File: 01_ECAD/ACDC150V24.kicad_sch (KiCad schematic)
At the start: 0 parts

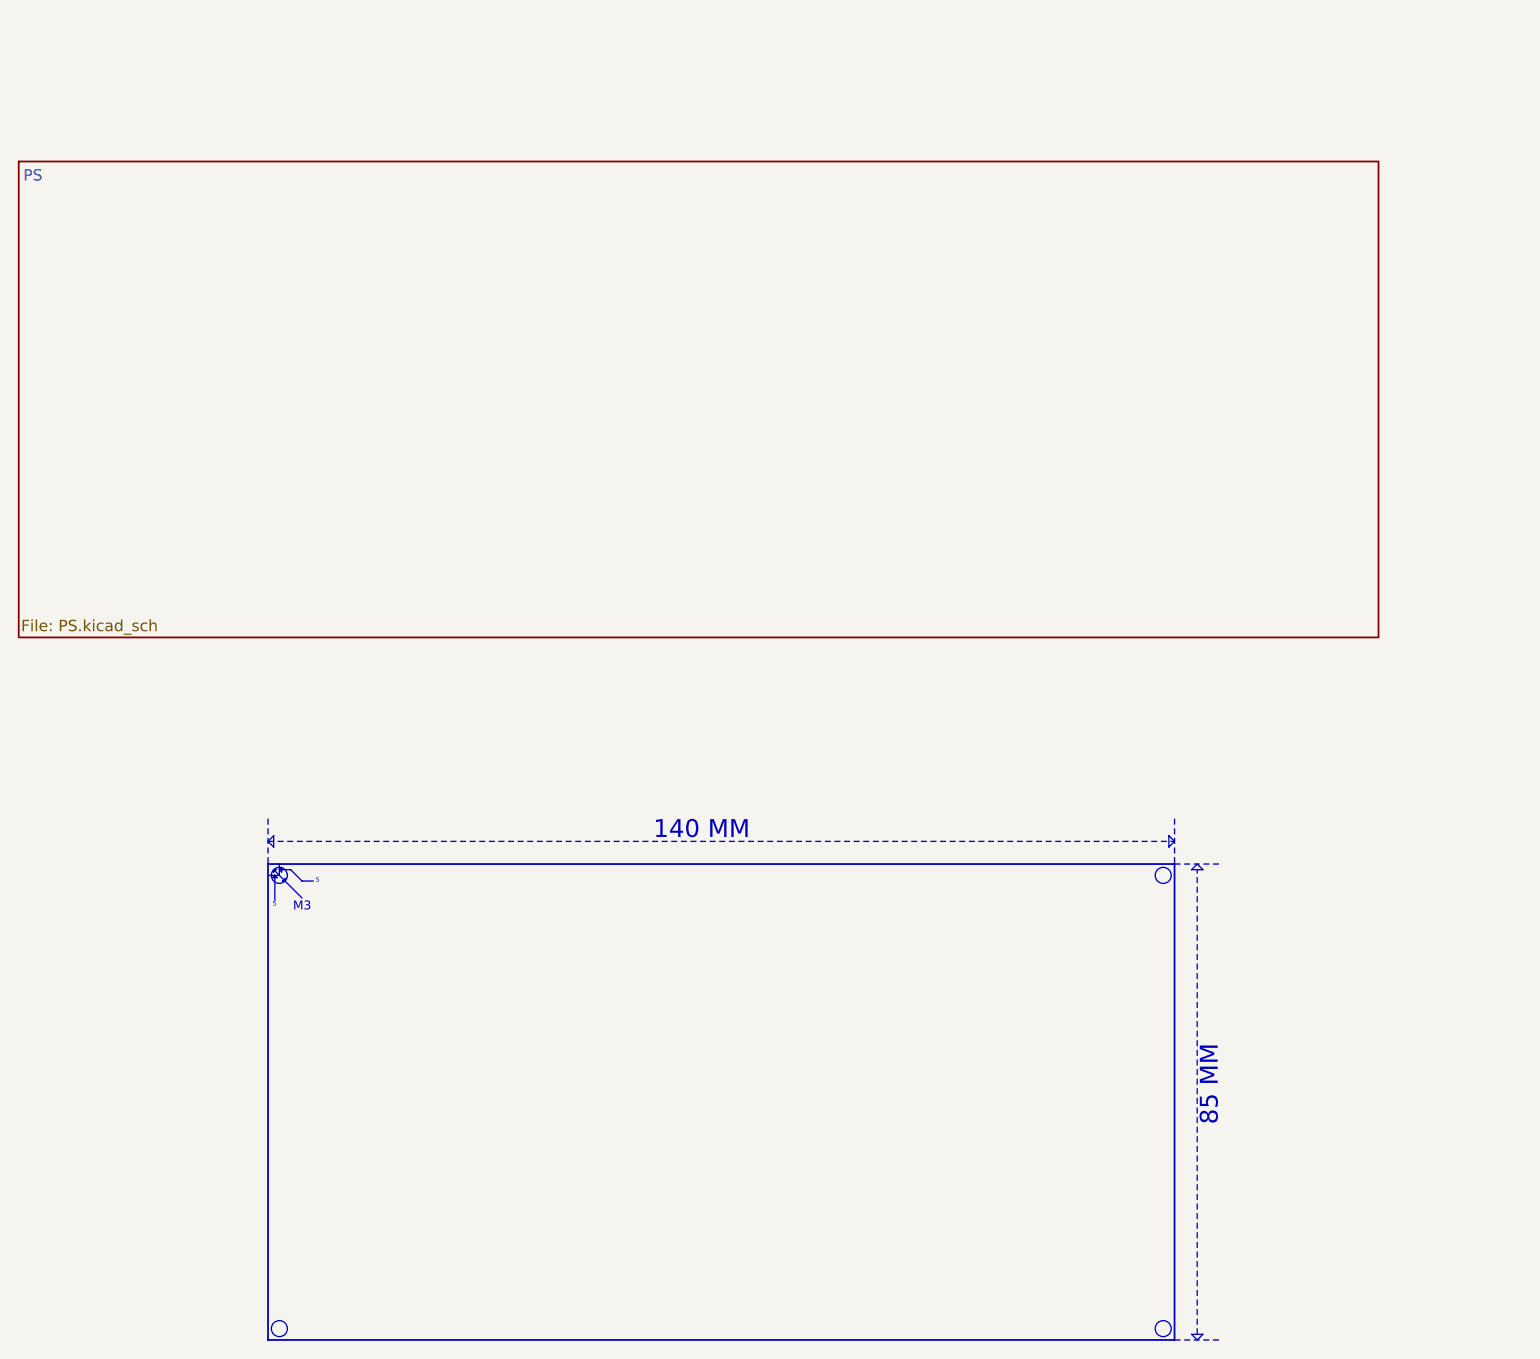
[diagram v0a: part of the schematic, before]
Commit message: Regular Update.
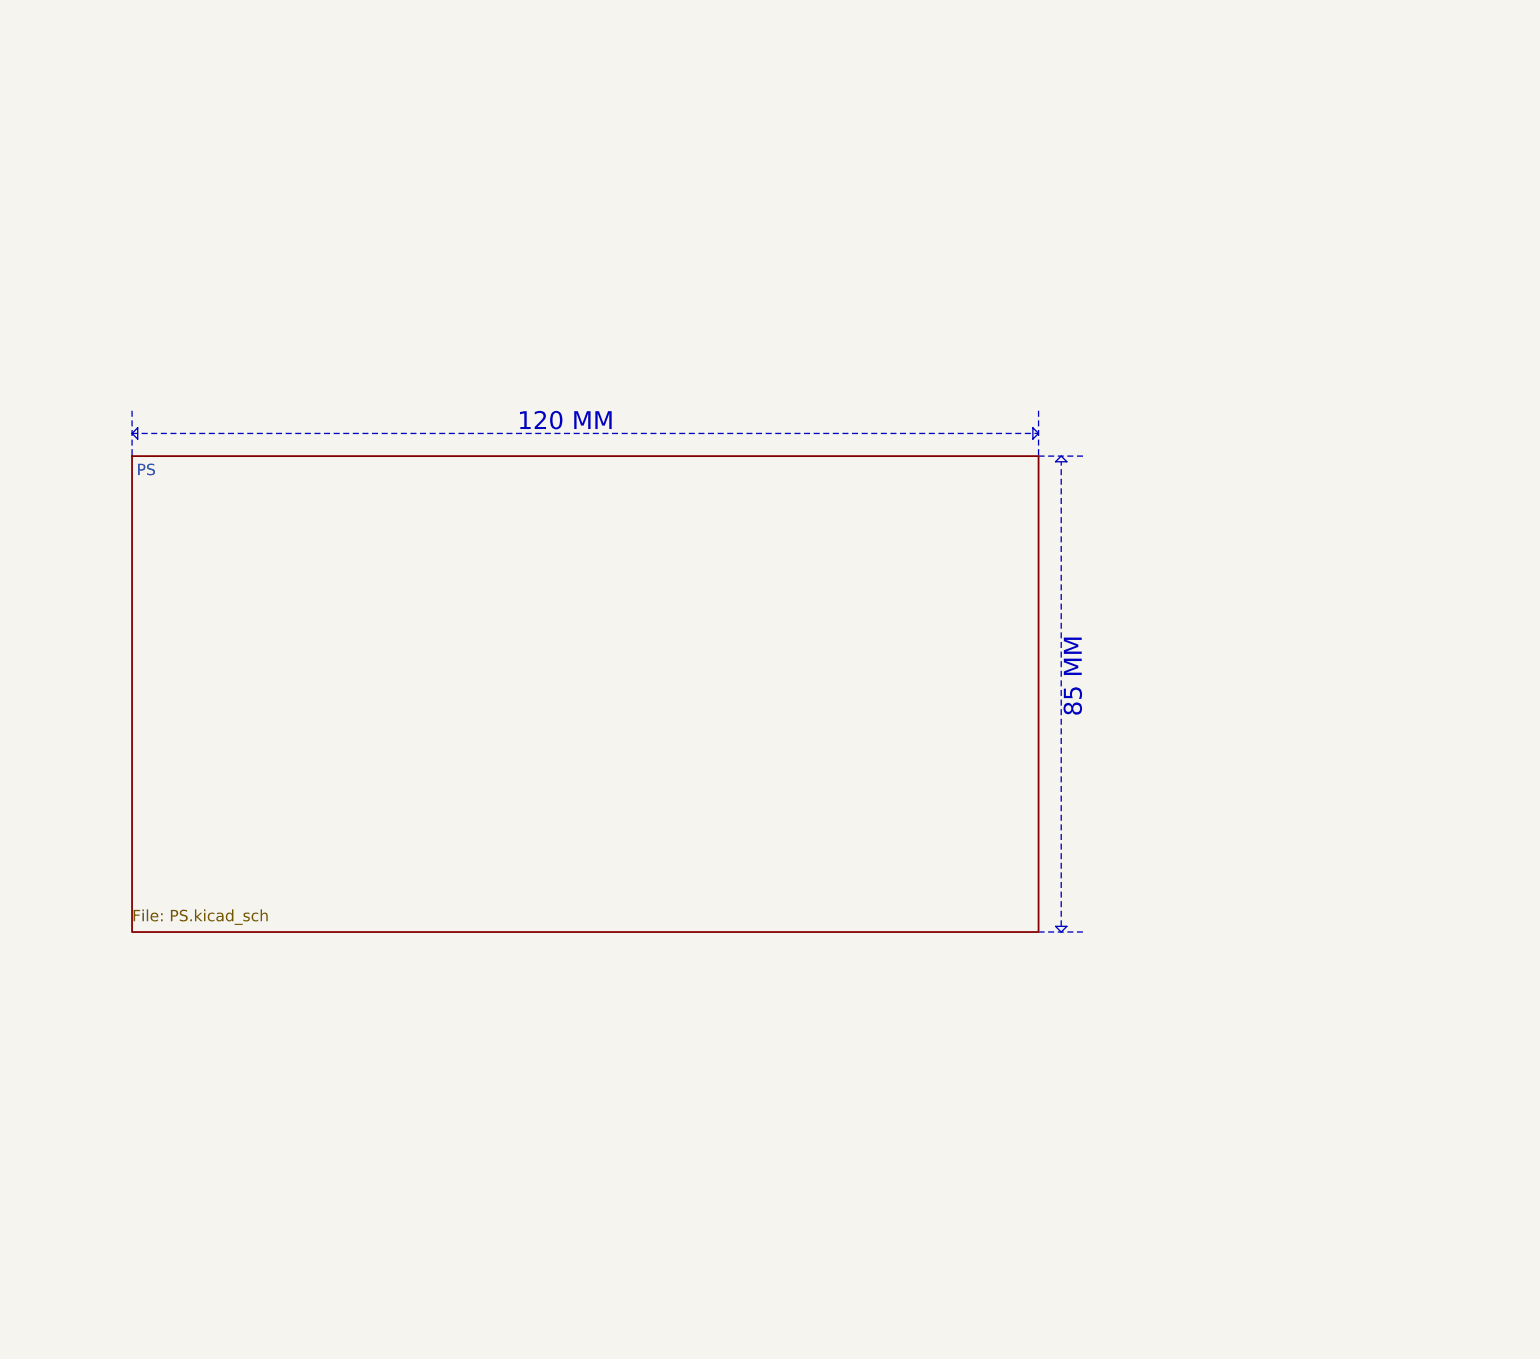
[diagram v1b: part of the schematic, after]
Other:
- note added: "120 MM"
- note removed: "140 MM"
- note removed: "5"
- note removed: "M3"
